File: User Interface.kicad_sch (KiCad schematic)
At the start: 4 parts, among them SW1 SW_DIP_x01, U1 7400, U2 7402

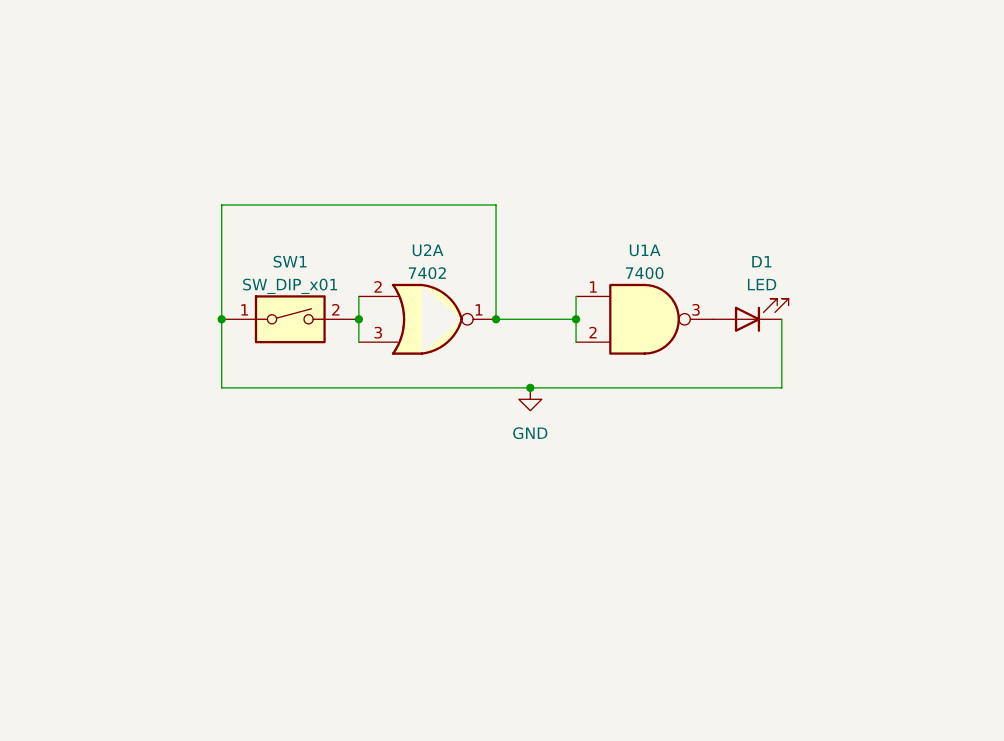
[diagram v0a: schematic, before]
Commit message: 3 How To Design A Circuit Using KiCad 7.0 Schematic Editor
https://www.youtube.com/watch?v=pgKfaFI4T4Y
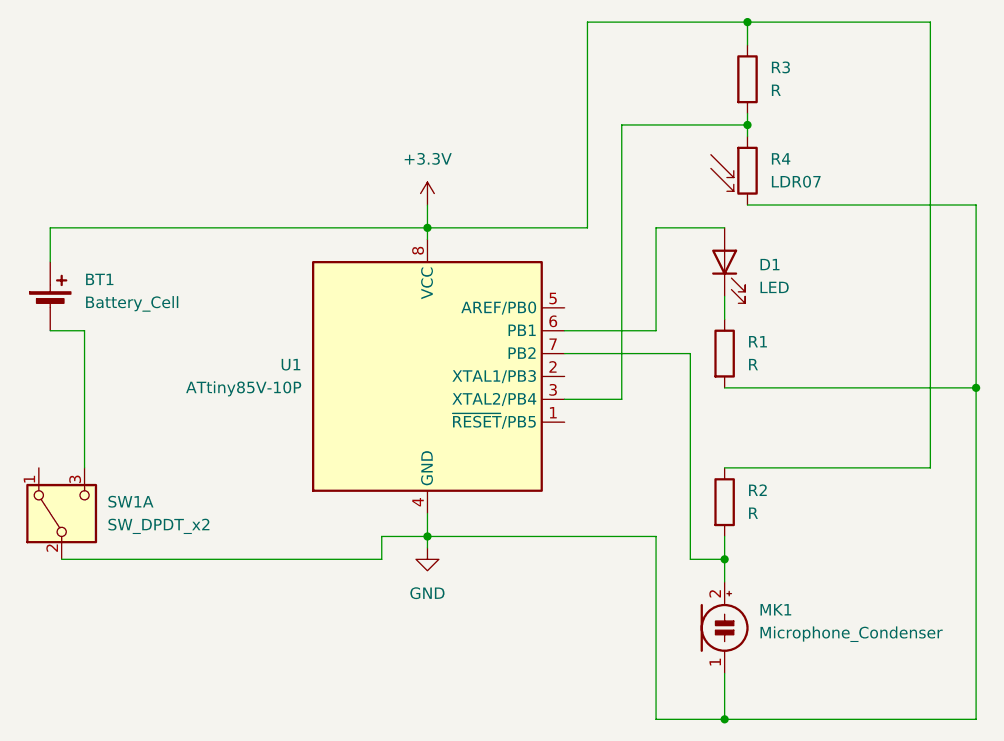
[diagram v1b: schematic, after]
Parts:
- removed SW1: SW_DIP_x01, symbol Switch:SW_DIP_x01
- removed U1: 7400, symbol 74xx:7400
- removed U2: 7402, symbol 74xx:7402
- added BT1: Battery_Cell, symbol Device:Battery_Cell
- added MK1: Microphone_Condenser, symbol Device:Microphone_Condenser
- added R1, R2, R3: R, symbol Device:R
- added R4: LDR07, OptoDevice:R_LDR_5.1x4.3mm_P3.4mm_Vertical, symbol Sensor_Optical:LDR07
- added SW1: SW_DPDT_x2, symbol Switch:SW_DPDT_x2
- added U1: ATtiny85V-10P, Package_DIP:DIP-8_W7.62mm, symbol MCU_Microchip_ATtiny:ATtiny85V-10P
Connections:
- net GND: now also MK1.1 (-), R1.2, R4.2, SW1.2 (B), U1.4 (GND); no longer D1.1 (K)
- net at D1.2 (A): now also U1.6 (PB1)
- new net: D1.1 (K), R1.1
- new net: MK1.2 (+), R2.2, U1.7 (PB2)
- new net: R3.2, R4.1, U1.3 (XTAL2/PB4)
- new net: BT1.2 (-), SW1.3 (C)
- new net +3.3V: BT1.1 (+), R2.1, R3.1, U1.8 (VCC)
